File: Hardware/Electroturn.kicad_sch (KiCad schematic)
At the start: 10 parts

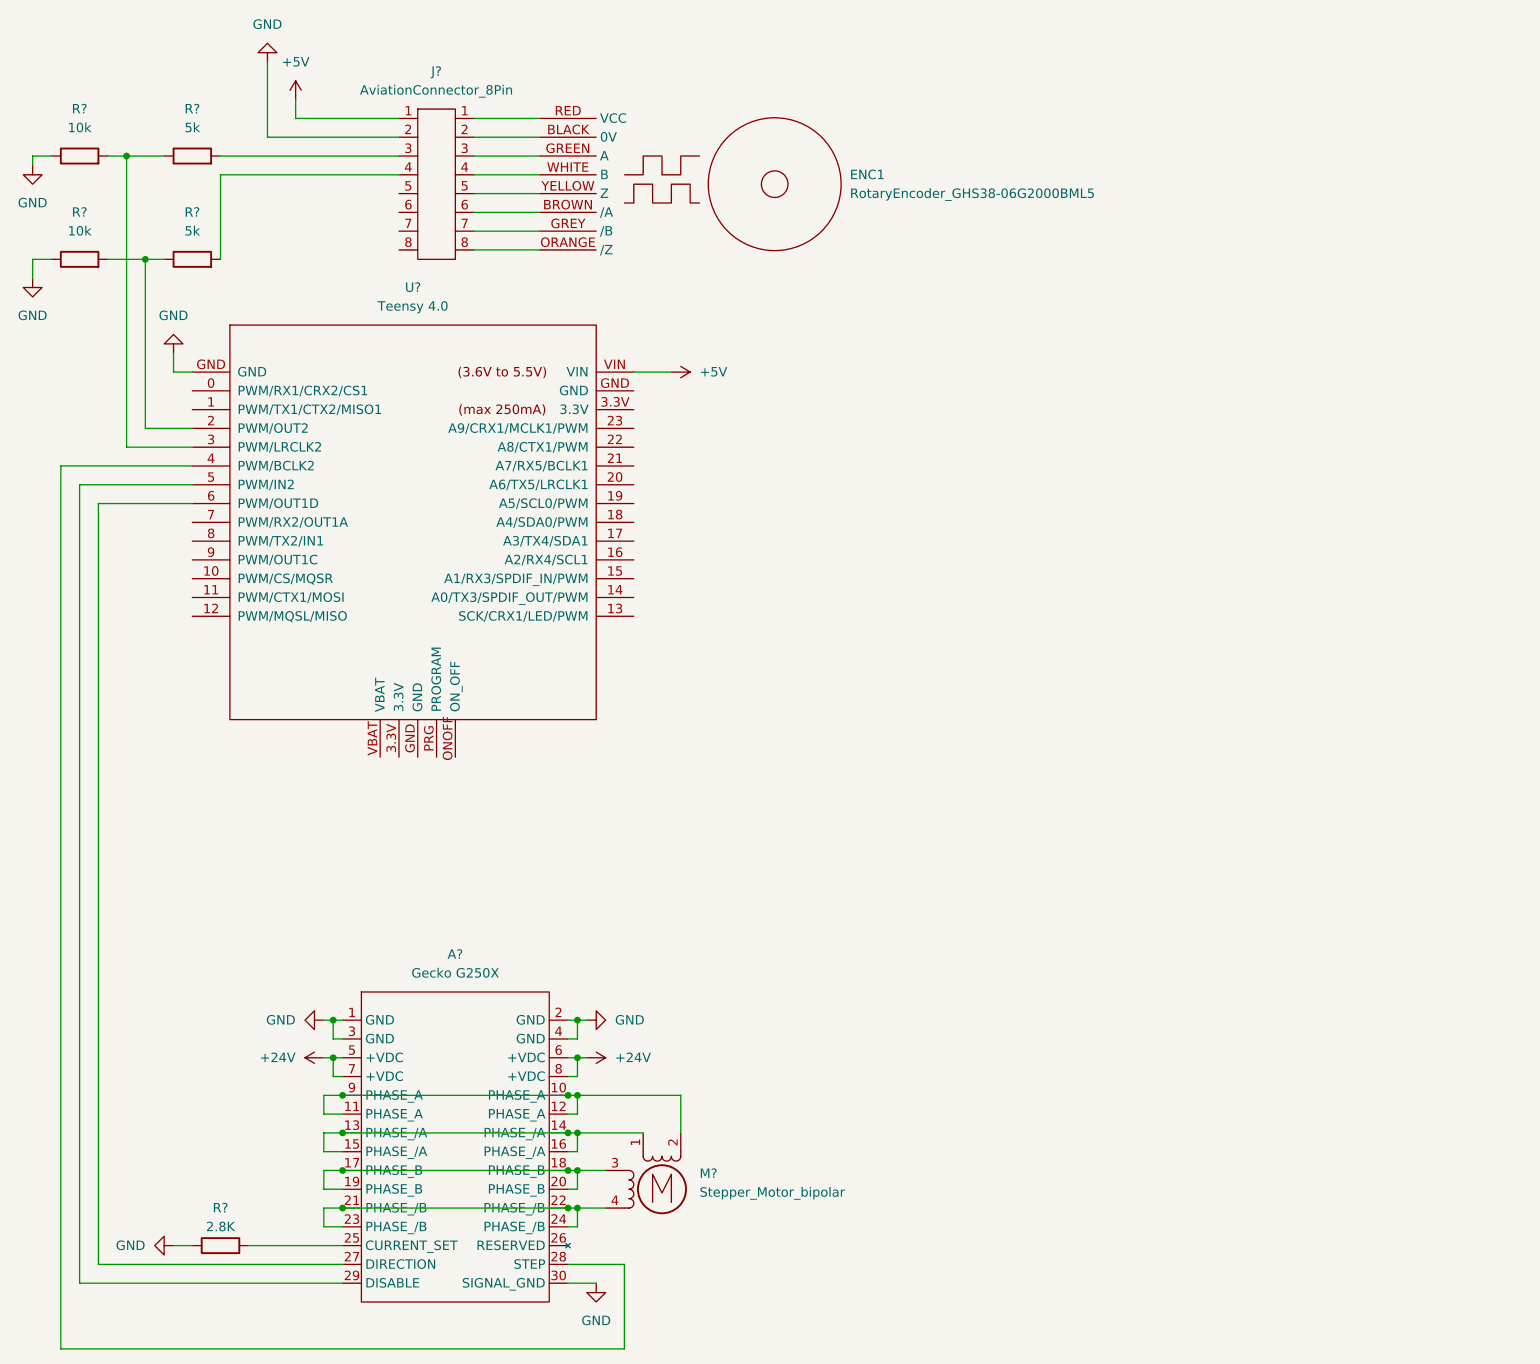
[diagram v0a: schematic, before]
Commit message: Beth Annes kicad work part 1
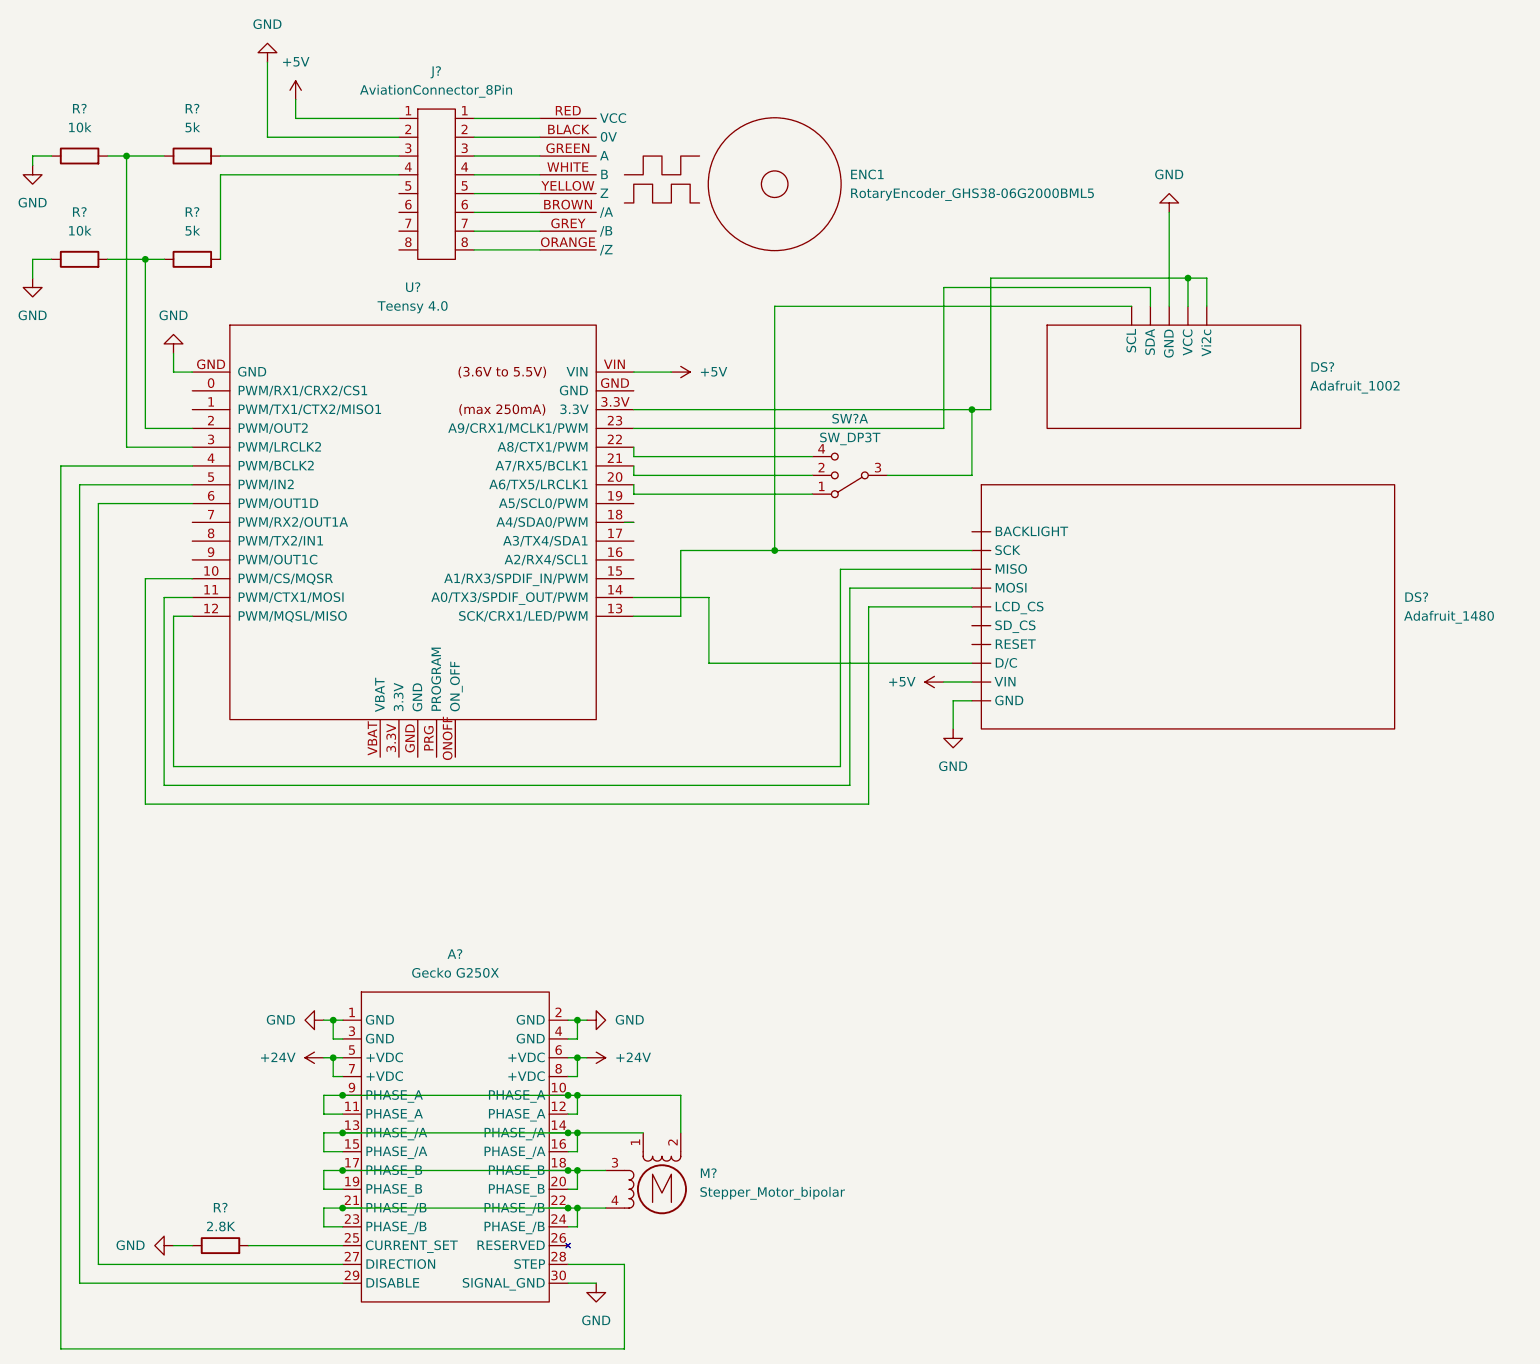
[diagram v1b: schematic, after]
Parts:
- added DS?: Adafruit_1480, symbol MCU_Module:Adafruit_1480
- added DS?: Adafruit_1002, symbol MCU_Module:Adafruit_1002
- added SW?: SW_DP3T, symbol Switch:SW_DP3T
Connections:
- net +5V: now also DS?. (VIN)
- net GND: now also DS?. (VIN), DS?. (Vi2c)
- net at U?.10 (PWM/CS/MQSR): now also DS?. (VIN)
- net at U?.11 (PWM/CTX1/MOSI): now also DS?. (VIN)
- net at U?.12 (PWM/MQSL/MISO): now also DS?. (VIN)
- net at U?.13 (SCK/CRX1/LED/PWM): now also DS?. (VIN), DS?. (Vi2c)
- net at U?.14 (A0/TX3/SPDIF_OUT/PWM): now also DS?. (VIN)
- net at U?.20 (A6/TX5/LRCLK1): now also SW?.1
- net at U?.21 (A7/RX5/BCLK1): now also SW?.2
- net at U?.22 (A8/CTX1/PWM): now also SW?.4
- net at U?.23 (A9/CRX1/MCLK1/PWM): now also DS?. (Vi2c)
- net at U?.3.3V: now also DS?. (Vi2c), SW?.3
